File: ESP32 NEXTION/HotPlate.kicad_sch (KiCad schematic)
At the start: 56 parts, among them J1 Barrel_Jack_Switch, J11 Conn_01x04_Male, J2 Conn_01x08_Male

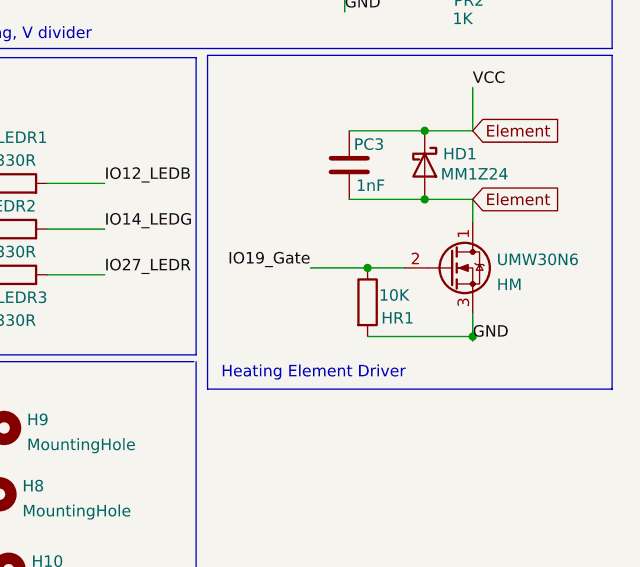
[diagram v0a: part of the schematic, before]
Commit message: revision 1.3
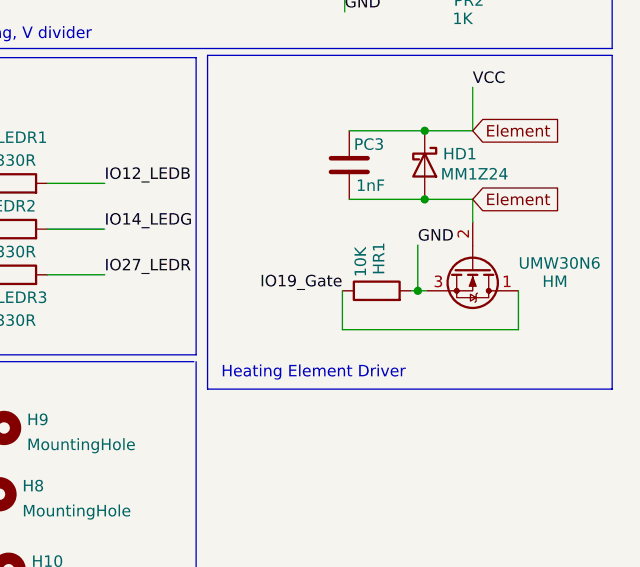
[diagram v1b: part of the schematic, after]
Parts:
- PC1: footprint Capacitor_SMD:CP_Elec_6.3x5.9 -> Capacitor_SMD:CP_Elec_10x12.5
- SMAJ18A1: footprint Diode_SMD:D_1210_3225Metric -> Diode_SMD:D_1210_3225Metric_Pad1.42x2.65mm_HandSolder
- UMW30N6: footprint Package_TO_SOT_SMD:TO-252-3_TabPin4 -> Package_TO_SOT_SMD:TO-252-2
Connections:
- net Element: now also UMW30N6.2 (G); no longer UMW30N6.1 (D)
- net IO19_Gate: now also UMW30N6.1 (D); no longer UMW30N6.2 (G)
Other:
- moved on the sheet: HR1, UMW30N6
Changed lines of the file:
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@@
   (junction (at 54.864 22.86) (diameter 0) (color 0 0 0 0)
   )
-  (junction (at 268.478 75.184) (diameter 0) (color 0 0 0 0)
-  )
   (junction (at 170.942 36.576) (diameter 0) (color 0 0 0 0)
   )
@@
   (junction (at 197.104 63.246) (diameter 0) (color 0 0 0 0)
   )
-  (junction (at 256.794 67.564) (diameter 0) (color 0 0 0 0)
-  )
   (junction (at 32.004 37.084) (diameter 0) (color 0 0 0 0)
   )
@@
   )
   (junction (at 82.296 47.244) (diameter 0) (color 0 0 0 0)
+  )
+  (junction (at 262.382 70.104) (diameter 0) (color 0 0 0 0)
   )
   (junction (at 263.144 59.944) (diameter 0) (color 0 0 0 0)
@@
   (no_connect (at 70.104 87.884))
   (no_connect (at 70.104 92.964))
-  (wire (pts (xy 256.794 75.184) (xy 268.478 75.184))
-    (stroke (width 0) (type default) (color 0 0 0 0))
-  )
   (polyline (pts (xy 192.532 134.62) (xy 192.532 114.046))
     (stroke (width 0) (type default) (color 0 0 0 0))
@@
     (stroke (width 0) (type default) (color 0 0 0 0))
   )
+  (wire (pts (xy 273.558 70.104) (xy 273.558 74.422))
+    (stroke (width 0) (type default) (color 0 0 0 0))
+  )
   (wire (pts (xy 251.46 140.97) (xy 251.46 143.764))
     (stroke (width 0) (type default) (color 0 0 0 0))
@@
     (stroke (width 0) (type default) (color 0 0 0 0))
   )
-  (wire (pts (xy 268.478 72.644) (xy 268.478 75.184))
-    (stroke (width 0) (type default) (color 0 0 0 0))
-  )
   (polyline (pts (xy 239.014 164.846) (xy 283.972 164.846))
     (stroke (width 0) (type default) (color 0 0 0 0))
@@
     (stroke (width 0) (type default) (color 0 0 0 0))
   )
+  (wire (pts (xy 254 70.104) (xy 254 74.422))
+    (stroke (width 0) (type default) (color 0 0 0 0))
+  )
   (wire (pts (xy 257.048 150.368) (xy 262.128 150.368))
     (stroke (width 0) (type default) (color 0 0 0 0))
@@
     (stroke (width 0) (type default) (color 0 0 0 0))
   )
-  (wire (pts (xy 250.444 67.564) (xy 256.794 67.564))
-    (stroke (width 0) (type default) (color 0 0 0 0))
-  )
   (wire (pts (xy 248.412 146.304) (xy 251.46 146.304))
     (stroke (width 0) (type default) (color 0 0 0 0))
@@
     (stroke (width 0) (type default) (color 0 0 0 0))
   )
+  (wire (pts (xy 254 74.422) (xy 273.558 74.422))
+    (stroke (width 0) (type default) (color 0 0 0 0))
+  )
   (wire (pts (xy 268.478 59.944) (xy 268.478 62.484))
     (stroke (width 0) (type default) (color 0 0 0 0))
@@
     (stroke (width 0) (type default) (color 0 0 0 0))
   )
+  (wire (pts (xy 262.382 70.104) (xy 263.398 70.104))
+    (stroke (width 0) (type default) (color 0 0 0 0))
+  )
+  (wire (pts (xy 262.382 65.024) (xy 262.382 70.104))
+    (stroke (width 0) (type default) (color 0 0 0 0))
+  )
   (wire (pts (xy 254.254 35.306) (xy 254.254 39.116))
     (stroke (width 0) (type default) (color 0 0 0 0))
@@
     (stroke (width 0) (type default) (color 0 0 0 0))
   )
+  (wire (pts (xy 261.62 70.104) (xy 262.382 70.104))
+    (stroke (width 0) (type default) (color 0 0 0 0))
+  )
   (wire (pts (xy 27.178 148.336) (xy 45.974 148.336))
     (stroke (width 0) (type default) (color 0 0 0 0))
@@
     (stroke (width 0) (type default) (color 0 0 0 0))
   )
-  (wire (pts (xy 268.478 75.184) (xy 268.478 75.692))
-    (stroke (width 0) (type default) (color 0 0 0 0))
-  )
   (wire (pts (xy 71.882 150.876) (xy 65.024 150.876))
     (stroke (width 0) (type default) (color 0 0 0 0))
@@
   )
   (wire (pts (xy 203.454 68.326) (xy 197.104 68.326))
-    (stroke (width 0) (type default) (color 0 0 0 0))
-  )
-  (wire (pts (xy 256.794 67.564) (xy 260.858 67.564))
     (stroke (width 0) (type default) (color 0 0 0 0))
   )
@@
     (effects (font (size 1.27 1.27)) (justify left bottom))
   )
-  (label "GND" (at 268.478 75.692 0)
+  (label "GND" (at 262.382 65.024 0)
     (effects (font (size 1.27 1.27)) (justify left bottom))
   )
@@
     (effects (font (size 1.27 1.27)) (justify left bottom))
   )
-  (label "IO19_Gate" (at 250.444 67.564 180)
+  (label "IO19_Gate" (at 254 70.104 180)
     (effects (font (size 1.27 1.27)) (justify right bottom))
   )
@@
       (effects (font (size 1.27 1.27)) (justify left))
     )
-    (property "Footprint" "Capacitor_SMD:CP_Elec_6.3x5.9" (id 2) (at 236.1692 30.48 0)
+    (property "Footprint" "Capacitor_SMD:CP_Elec_10x12.5" (id 2) (at 236.1692 30.48 0)
       (effects (font (size 1.27 1.27)) hide)
     )
@@
       (effects (font (size 1.27 1.27)) (justify right))
     )
-    (property "Footprint" "Diode_SMD:D_1210_3225Metric" (id 2) (at 226.568 27.178 0)
+    (property "Footprint" "Diode_SMD:D_1210_3225Metric_Pad1.42x2.65mm_HandSolder" (id 2) (at 226.568 27.178 0)
       (effects (font (size 1.27 1.27)) hide)
     )
@@
     (pin "2")
   )
-  (symbol (lib_id "Device:R") (at 256.794 71.374 0) (unit 1)
-    (in_bom yes) (on_board yes)
-    (property "Reference" "HR1" (id 0) (at 258.318 73.152 0)
-      (effects (font (size 1.27 1.27)) (justify left))
-    )
-    (property "Value" "10K" (id 1) (at 258.064 70.612 0)
-      (effects (font (size 1.27 1.27)) (justify left))
-    )
-    (property "Footprint" "Capacitor_SMD:C_1206_3216Metric_Pad1.33x1.80mm_HandSolder" (id 2) (at 255.016 71.374 90)
-      (effects (font (size 1.27 1.27)) hide)
-    )
-    (property "Datasheet" "~" (id 3) (at 256.794 71.374 0)
+  (symbol (lib_id "Device:R") (at 257.81 70.104 90) (unit 1)
+    (in_bom yes) (on_board yes)
+    (property "Reference" "HR1" (id 0) (at 258.064 68.326 0)
+      (effects (font (size 1.27 1.27)) (justify left))
+    )
+    (property "Value" "10K" (id 1) (at 256.032 68.58 0)
+      (effects (font (size 1.27 1.27)) (justify left))
+    )
+    (property "Footprint" "Capacitor_SMD:C_1206_3216Metric_Pad1.33x1.80mm_HandSolder" (id 2) (at 257.81 71.882 90)
+      (effects (font (size 1.27 1.27)) hide)
+    )
+    (property "Datasheet" "~" (id 3) (at 257.81 70.104 0)
       (effects (font (size 1.27 1.27)) hide)
     )
@@
     (pin "2")
   )
-  (symbol (lib_id "Device:Q_NMOS_DGS") (at 265.938 67.564 0) (unit 1)
-    (in_bom yes) (on_board yes) (fields_autoplaced)
-    (property "Reference" "UMW30N6" (id 0) (at 271.145 66.6555 0)
-      (effects (font (size 1.27 1.27)) (justify left))
-    )
-    (property "Value" "HM" (id 1) (at 271.145 69.4306 0)
-      (effects (font (size 1.27 1.27)) (justify left))
-    )
-    (property "Footprint" "Package_TO_SOT_SMD:TO-252-3_TabPin4" (id 2) (at 271.018 65.024 0)
-      (effects (font (size 1.27 1.27)) hide)
-    )
-    (property "Datasheet" "~" (id 3) (at 265.938 67.564 0)
+  (symbol (lib_id "Device:Q_NMOS_DGS") (at 268.478 67.564 270) (unit 1)
+    (in_bom yes) (on_board yes)
+    (property "Reference" "UMW30N6" (id 0) (at 278.13 67.056 90))
+    (property "Value" "HM" (id 1) (at 277.622 69.088 90))
+    (property "Footprint" "Package_TO_SOT_SMD:TO-252-2" (id 2) (at 271.018 72.644 0)
+      (effects (font (size 1.27 1.27)) hide)
+    )
+    (property "Datasheet" "~" (id 3) (at 268.478 67.564 0)
       (effects (font (size 1.27 1.27)) hide)
     )
@@
     )
     (path "/04997c0e-f533-4da3-8aed-3484d2569925"
-      (reference "PC1") (unit 1) (value "100uF") (footprint "Capacitor_SMD:CP_Elec_6.3x5.9")
+      (reference "PC1") (unit 1) (value "100uF") (footprint "Capacitor_SMD:CP_Elec_10x12.5")
     )
     (path "/43452d5b-ba44-4473-b7ed-b0e4c7902559"
@@
     )
     (path "/737c3eb0-edd7-42a7-b782-07a107f00a56"
-      (reference "SMAJ18A1") (unit 1) (value "SMAJ18A") (footprint "Diode_SMD:D_1210_3225Metric")
+      (reference "SMAJ18A1") (unit 1) (value "SMAJ18A") (footprint "Diode_SMD:D_1210_3225Metric_Pad1.42x2.65mm_HandSolder")
     )
     (path "/8fb3f598-be1a-4928-9caf-76ce6e9fe6e3"
@@
     )
     (path "/ca0239ea-7847-4675-adb8-634cbeec5b9a"
-      (reference "UMW30N6") (unit 1) (value "HM") (footprint "Package_TO_SOT_SMD:TO-252-3_TabPin4")
-    )
-  )
+      (reference "UMW30N6") (unit 1) (value "HM") (footprint "Package_TO_SOT_SMD:TO-252-2")
+    )
+  )
